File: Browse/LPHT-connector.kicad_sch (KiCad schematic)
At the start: 5 parts, among them J7 LPHT-04-16-L-RT1-GP

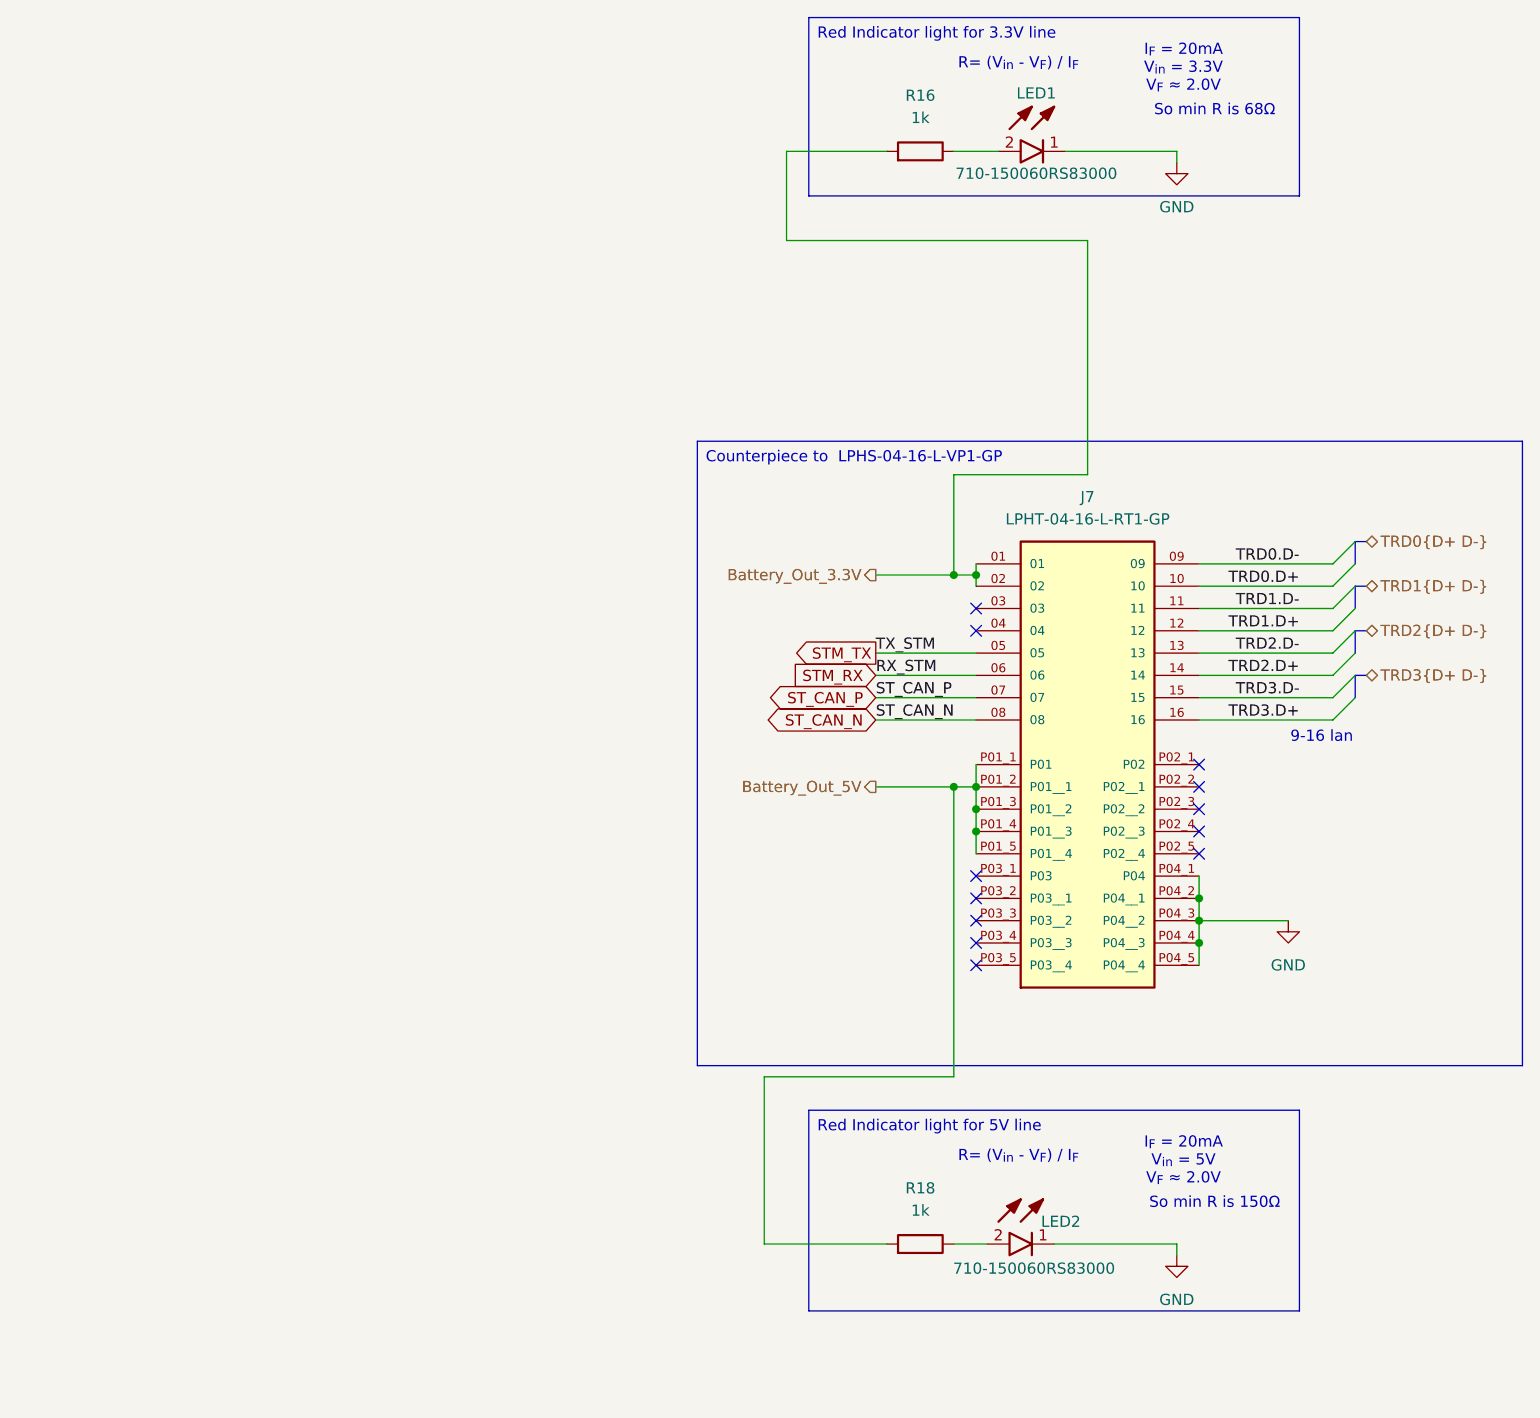
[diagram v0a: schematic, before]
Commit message: Deploying to gh-pages from @ Nautilus-UUV/nautilus-mainboard-PCB@5b07cf6af03655ef9ddad269b1edd5eb03bfa75f 🚀
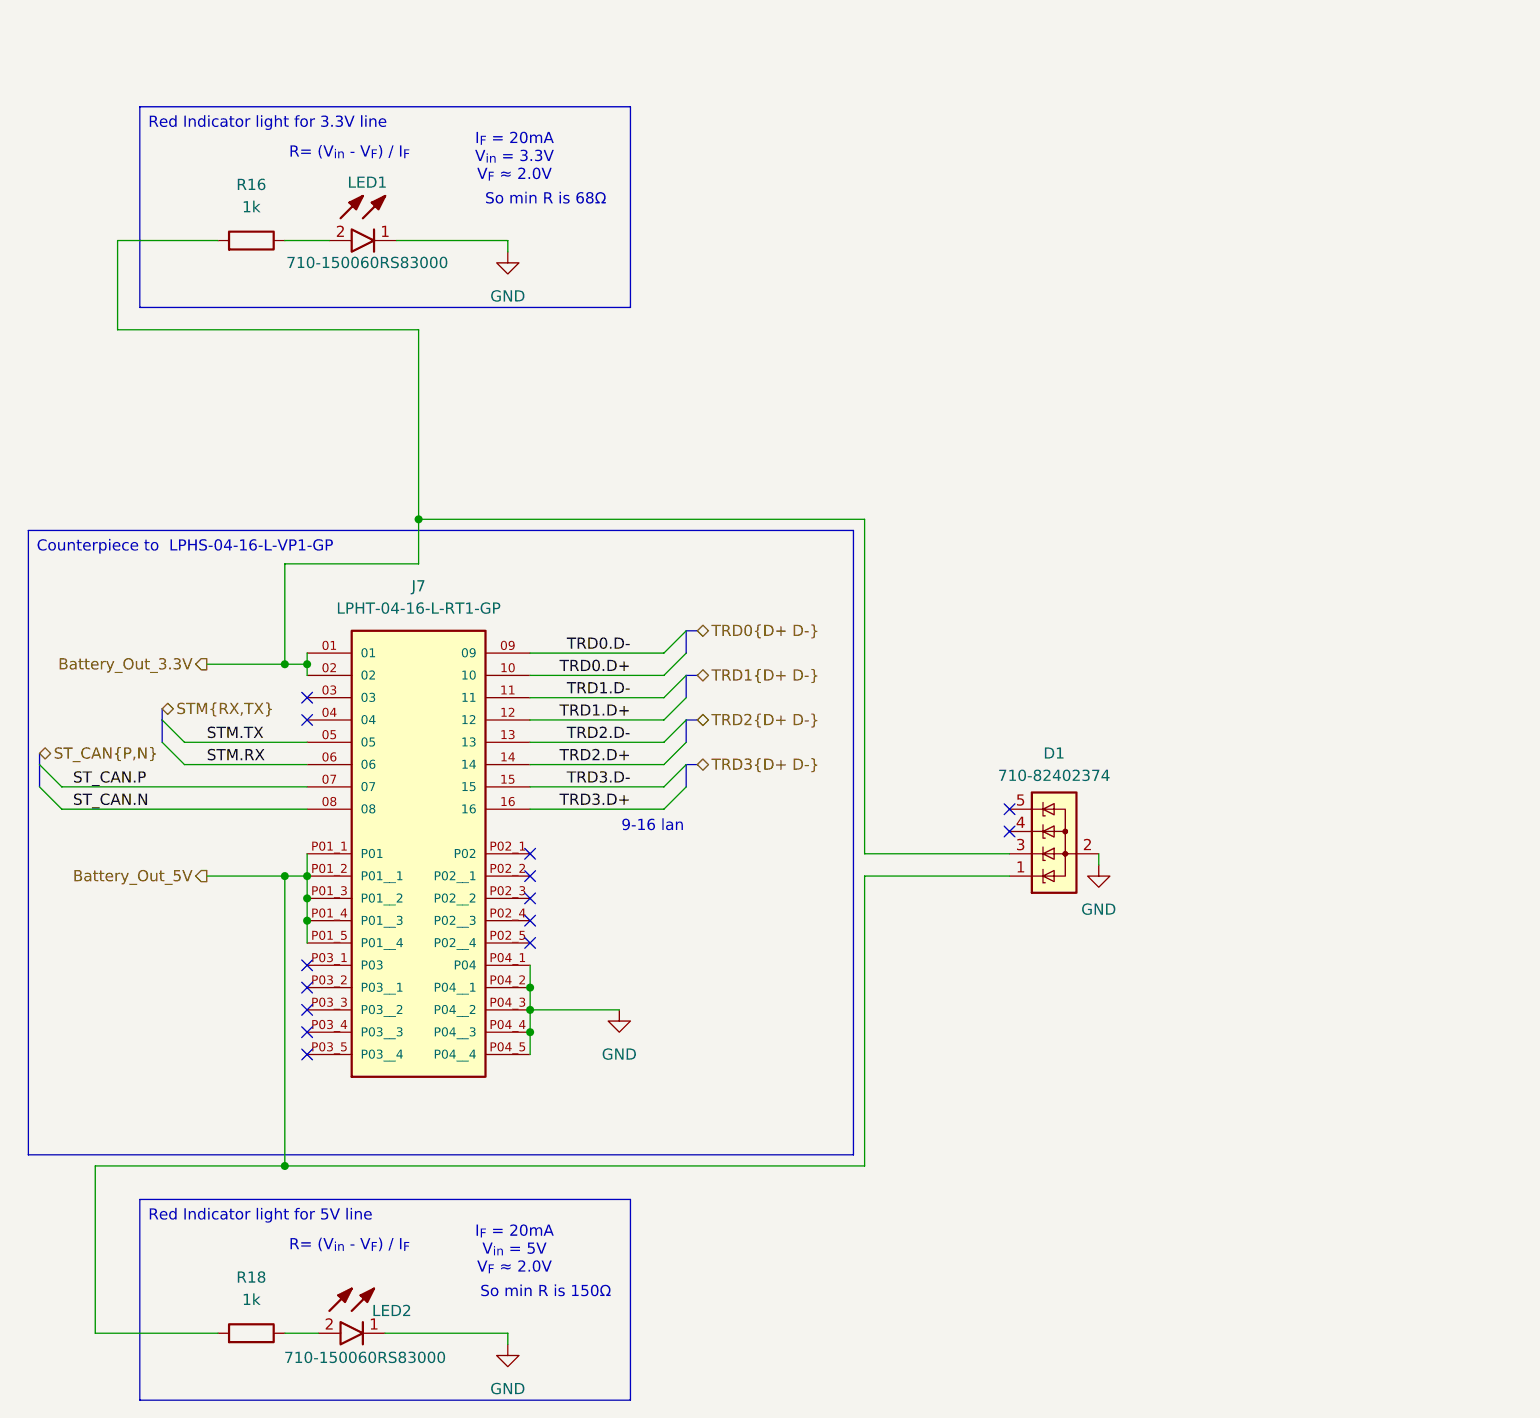
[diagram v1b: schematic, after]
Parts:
- added D1: 710-82402374, Package_TO_SOT_SMD:SOT-23-5, symbol #dzdb:s_dio/WURT-710-82402374
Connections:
- net Battery_Out_3.3V: now also D1.3 (K)
- net Battery_Out_5V: now also D1.1 (K)
- net GND: now also D1.2 (A)
- net STM_RX renamed STM.RX
- net STM_TX renamed STM.TX
- net ST_CAN_N renamed ST_CAN.N
- net ST_CAN_P renamed ST_CAN.P
- no-connect marks 12 -> 14
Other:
- title: (none) -> Nautilus_Mainboard
- moved on the sheet: J7, LED1, LED2, R16, R18
